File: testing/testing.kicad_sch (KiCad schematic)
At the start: 3 parts

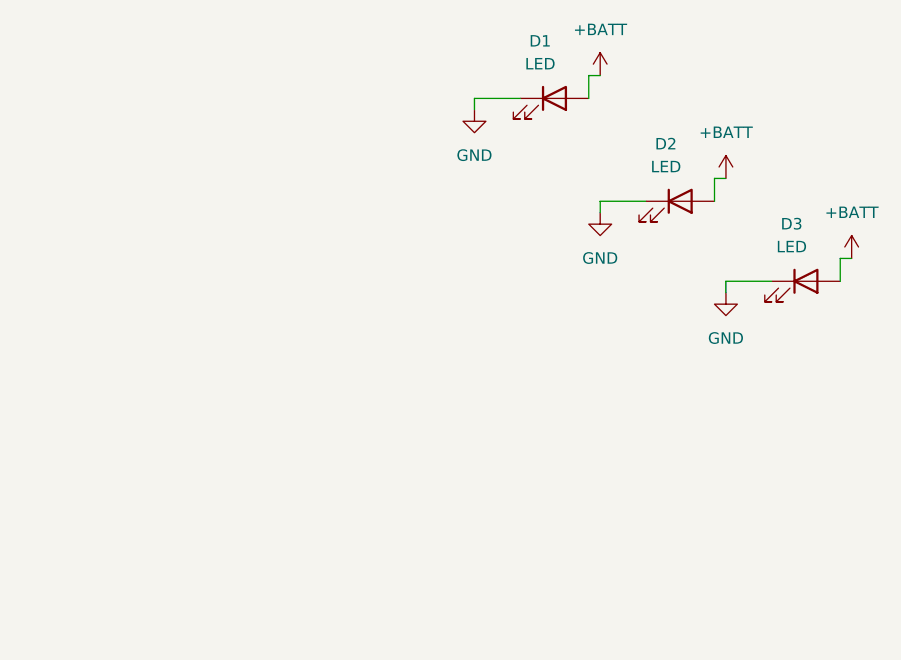
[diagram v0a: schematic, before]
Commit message: Testing Commit 12
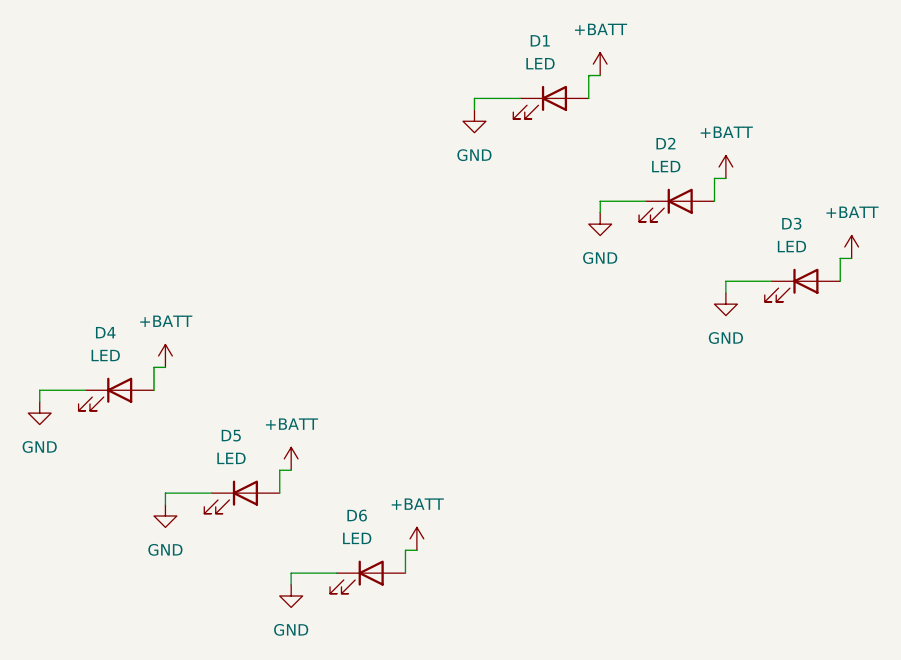
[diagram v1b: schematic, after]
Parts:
- added D4, D5, D6: LED, symbol Device:LED
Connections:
- net +BATT: now also D4.2 (A), D5.2 (A), D6.2 (A)
- net GND: now also D4.1 (K), D5.1 (K), D6.1 (K)

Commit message: Test Commit 13
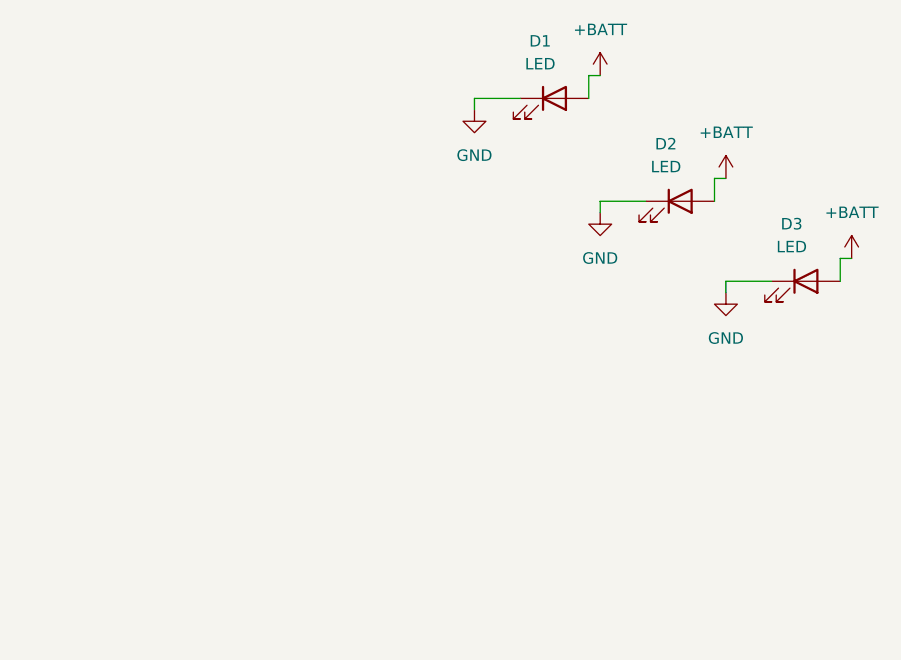
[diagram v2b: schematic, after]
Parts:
- removed D4, D5, D6: LED, symbol Device:LED
